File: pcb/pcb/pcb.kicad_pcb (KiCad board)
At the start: 2 copper layers, 28 parts, among them J1 SD Card, J2 Mic, J3 Relay Solenoid, J4 Status LED, P1 Power, SW1 Button Up, SW2 Button Down, SW3 Button Record, SW4 Button Delete, SW5 Button Play

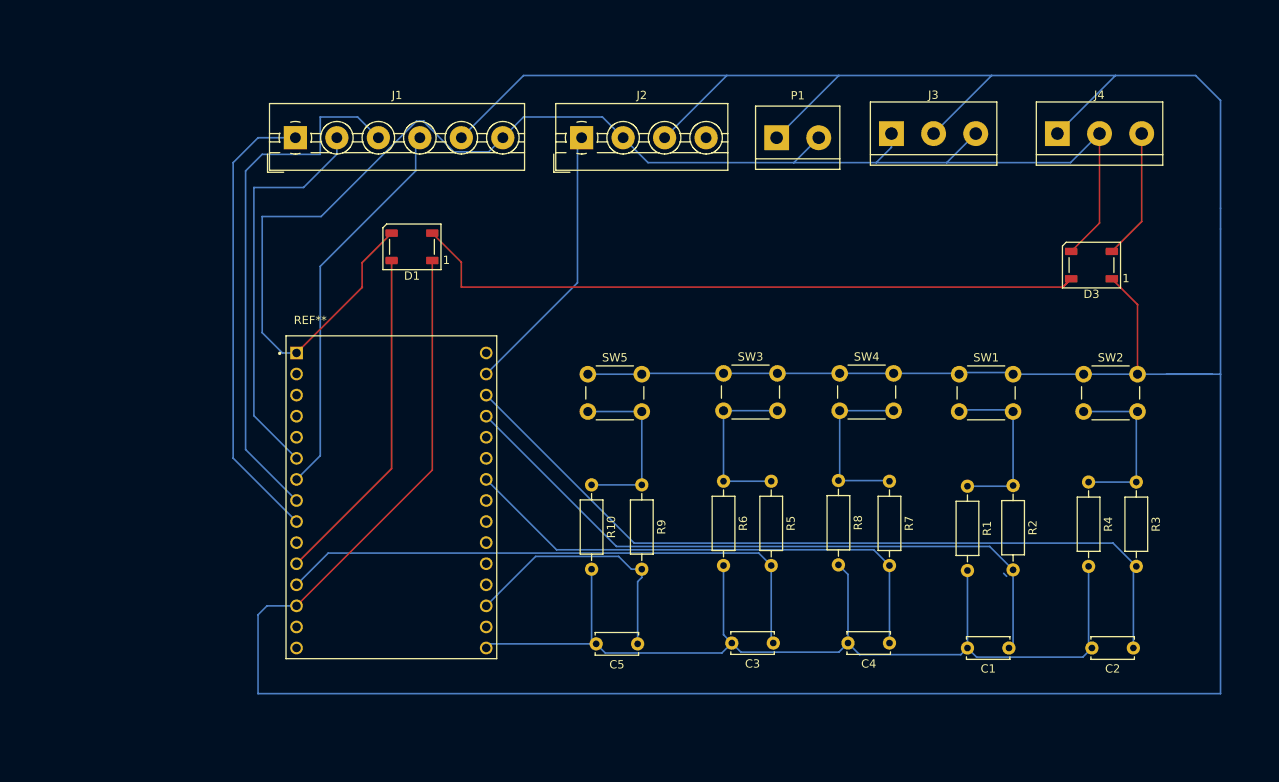
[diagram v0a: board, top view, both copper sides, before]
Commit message: PCB-Update
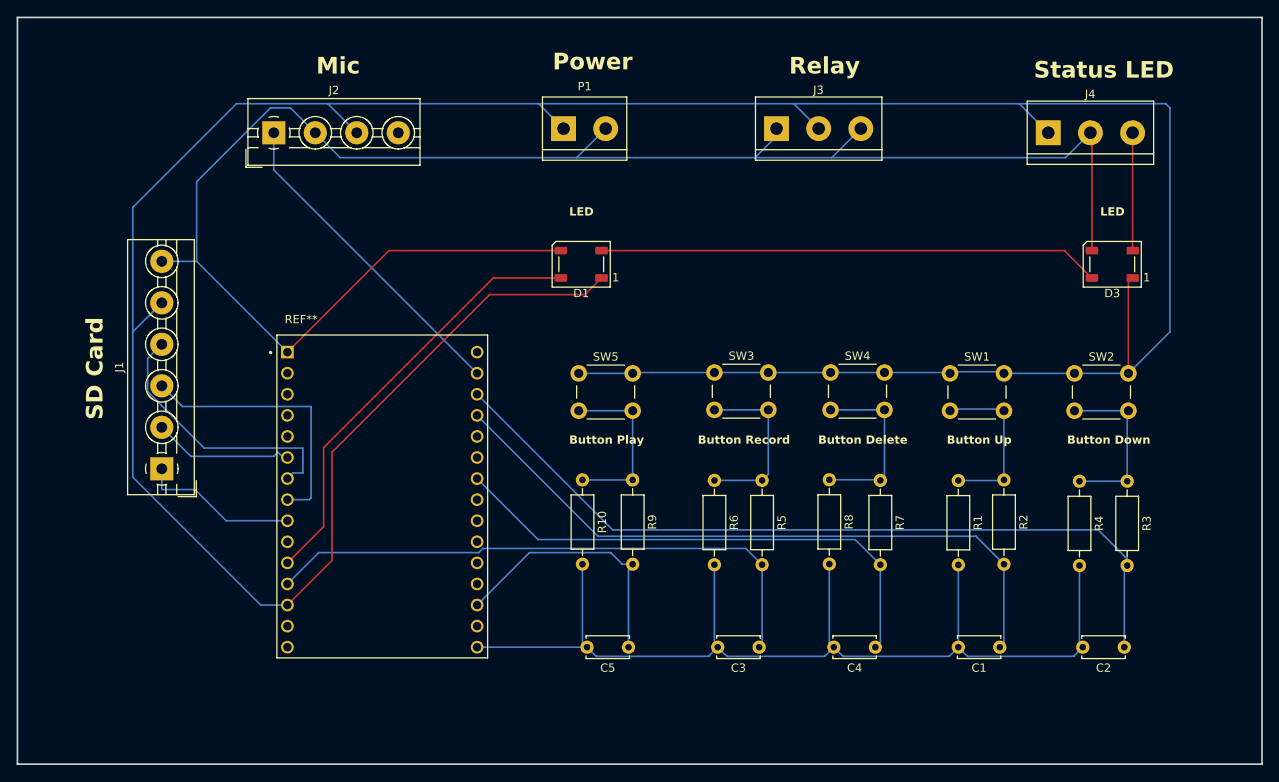
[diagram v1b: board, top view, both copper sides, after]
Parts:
- moved J1 43.0 mm to (80.4, 104.9), turned to 90 degrees
- moved J2 37.1 mm to (93.9, 64.4)
- moved P1 25.7 mm to (128.8, 63.9)
- moved D1 20.5 mm to (130.9, 80.2)
- moved J3 13.9 mm to (154.5, 63.9)
- moved D3 2.50 mm to (194.9, 80.2)
- moved C3 1.77 mm to (152.4, 126.4)
- moved C4 1.77 mm to (166.4, 126.4)
- moved R1 1.29 mm to (176.4, 106.3)
- moved R2 1.29 mm to (181.9, 106.2)
- moved R10 1.25 mm to (131.1, 106.2)
- moved R9 1.25 mm to (137.2, 106.2)
- moved C5 1.17 mm to (136.7, 126.4)
- moved R5 1.10 mm to (152.8, 106.3)
- moved R6 1.10 mm to (147.0, 106.3)
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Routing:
- net 5V: track 482.1 -> 385.3 mm
- net Net-(J1-CS): track 55.2 -> 19.2 mm
- net GND: track 306.5 -> 339.5 mm
- net Net-(J1-MOSI): track 64.6 -> 33.0 mm
- net Net-(J1-SCK): track 48.4 -> 17.1 mm
- net Net-(D1-DOUT): track 83.4 -> 60.5 mm
- net Net-(J1-MISO): track 47.3 -> 33.1 mm
- net Net-(D1-DIN): track 41.3 -> 52.8 mm
- net Net-(J2-A0): track 33.2 -> 39.8 mm
- net Net-(U1-GPIO19/USBD_+): track 31.1 -> 32.9 mm
- net Net-(D3-DOUT): track 15.7 -> 14.2 mm
- net Net-(U1-GPIO9): track 68.9 -> 70.2 mm
- net Net-(U1-GPIO10): track 62.2 -> 63.1 mm
- net Net-(R1-Pad1): track 21.0 -> 20.4 mm
- net (no net): track 0.51 -> 0.00 mm
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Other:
- board outline added: 150 x 90 mm
- board text added: "Button Delete"
- board text added: "Button Down"
- board text added: "Button Play"
- board text added: "Button Record"
- board text added: "Button Up"
- board text added: "LED"
- board text added: "Mic"
- board text added: "Power"
- board text added: "Relay"
- board text added: "SD Card"
- board text added: "Status LED"
